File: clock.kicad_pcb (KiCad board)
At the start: 2 copper layers, 129 parts, among them J1 USB_C_Receptacle_USB2.0_16P, J3 Conn_01x02_Pin, J4 Conn_01x02_Pin, Q1 2N7002K, Q2 NPN, U1 STM32F072CBT6, U2 USBLC6-2SC6, U4 MCP73871-2CC, U5 AP2112K-3.3, Y1 8MHz

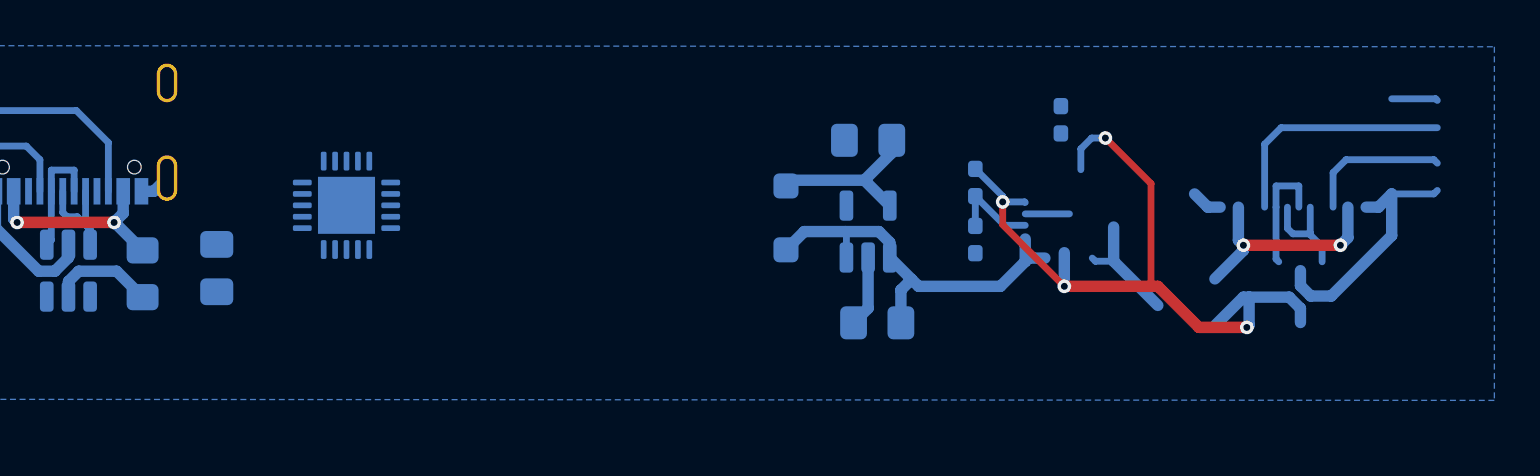
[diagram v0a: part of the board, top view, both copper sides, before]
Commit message: more routing
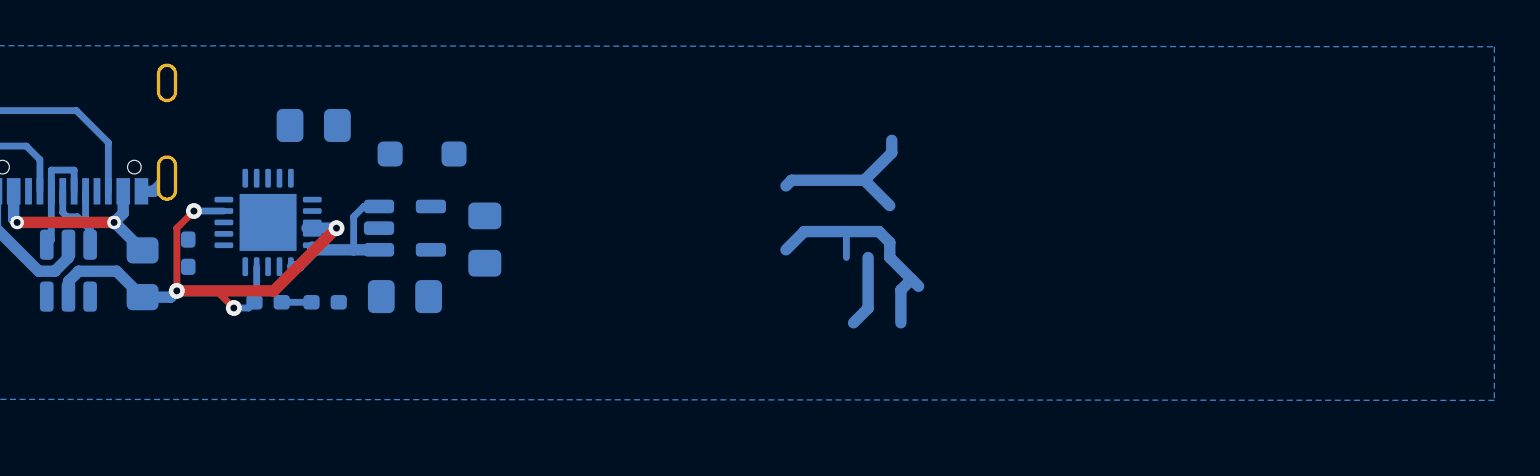
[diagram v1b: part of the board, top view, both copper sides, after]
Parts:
- moved R6 38.7 mm to (218.0, 35.3), turned to -90 degrees
- moved R10 31.4 mm to (221.5, 37.5), turned to 0 degrees
- moved R11 28.6 mm to (224.0, 37.5), turned to 180 degrees
- moved C18 20.7 mm to (227.5, 37.2), turned to 0 degrees
- moved U5 20.3 mm to (227.5, 34.2), turned to 0 degrees
- moved C19 17.4 mm to (231.0, 34.8), turned to -90 degrees
- moved D76 16.2 mm to (228.2, 31.0), turned to 0 degrees
- moved C17 7.56 mm to (223.5, 29.8), turned to 180 degrees
- moved U4 3.52 mm to (221.5, 34.0), turned to 90 degrees
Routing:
- net GND: track 33.7 -> 17.2 mm
- net +5V: track 38.7 -> 26.2 mm
- net Net-(J1-CC1): track 17.8 -> 7.13 mm
- net /VBUS: track 18.8 -> 8.97 mm, vias 4 -> 2
- net Net-(J1-CC2): track 17.6 -> 11.2 mm
- net D_BUS-: track 10.6 -> 5.28 mm
- net Net-(J5-Pin_1): track 5.23 -> 0.00 mm
- net D_BUS+: track 9.49 -> 4.86 mm
- net Net-(U4-VPCC): track 4.02 -> 1.31 mm
